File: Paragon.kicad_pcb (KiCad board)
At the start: 2 copper layers, 63 x 88 mm, 3 parts

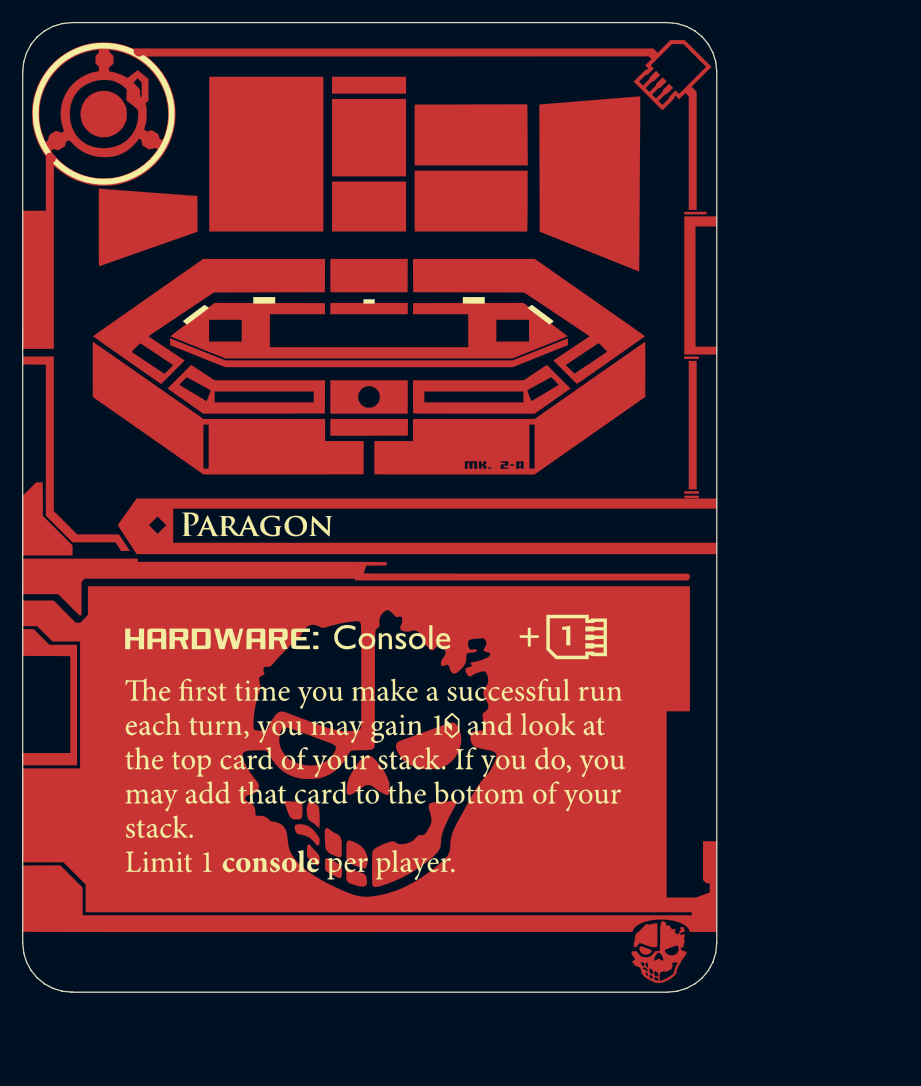
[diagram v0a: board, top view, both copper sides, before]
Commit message: Add files via upload
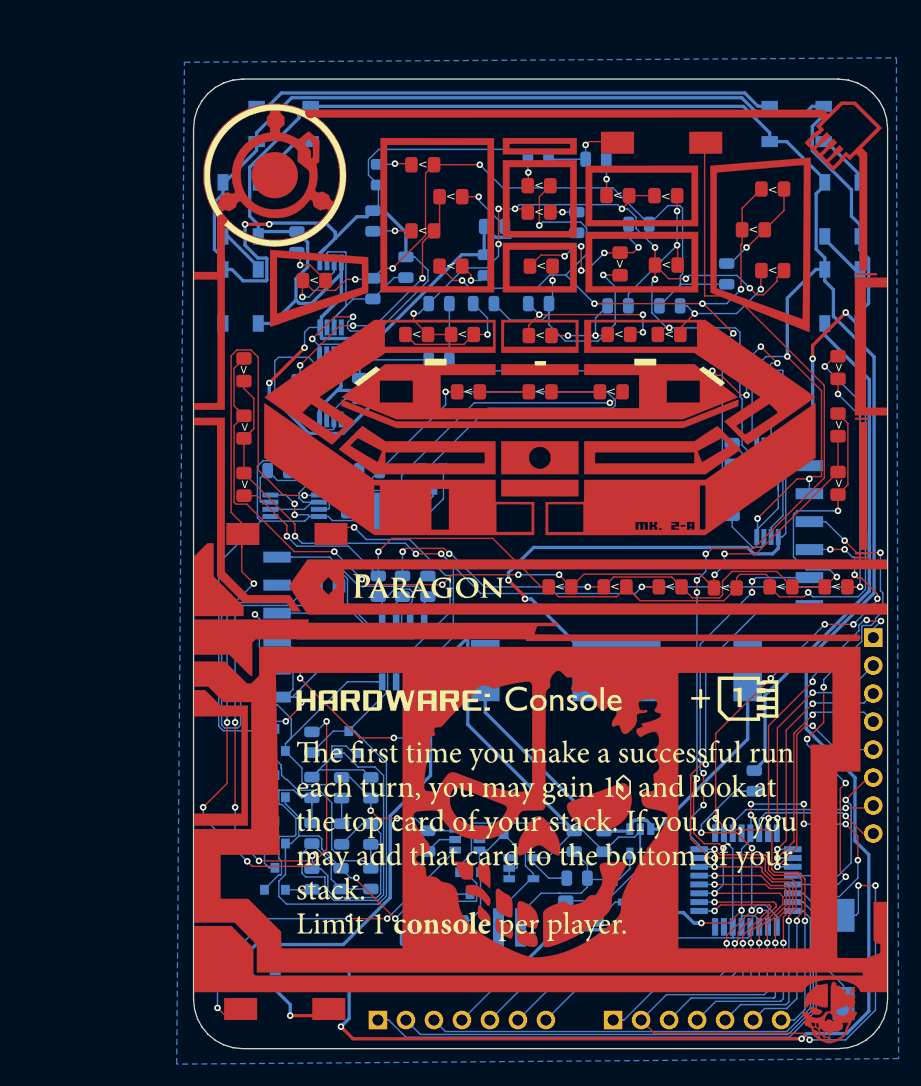
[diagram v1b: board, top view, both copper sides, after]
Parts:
- removed the G*** at (138.8, 93.2) (x2)
- removed the G*** at (138.8, 93.1)
- added 5551: NE555, Package_SO:TSSOP-8_4.4x3mm_P0.65mm, B.Cu at (135.3, 73.9)
- added 5552: NE555, Package_SO:TSSOP-8_4.4x3mm_P0.65mm, B.Cu at (135.2, 82.3)
- added 5553: NE555, Package_SO:TSSOP-8_4.4x3mm_P0.65mm, B.Cu at (174.9, 92.9)
- added 5554: NE555, Package_SO:TSSOP-8_4.4x3mm_P0.65mm, B.Cu at (174.9, 84.6)
- added AP2112: AP2112K-3.3, Package_TO_SOT_SMD:SOT-23-5, B.Cu at (163.0, 129.9)
- added ATA1: Conn_01x08_Male, KiCad Footprints:PinHeader_1x08_P2.54mm_Vertical, B.Cu at (184.5, 105.0)
- added ATD1: Conn_01x07_Male, KiCad Footprints:PinHeader_1x07_P2.54mm_Vertical, B.Cu at (139.6, 139.7)
- added ATD2: Conn_01x07_Male, KiCad Footprints:PinHeader_1x07_P2.54mm_Vertical, B.Cu at (160.9, 139.7)
- added ATM328: ATmega328P-AU, Package_QFP:TQFP-32_7x7mm_P0.8mm, B.Cu at (172.9, 127.0)
- added ATM328 SPI: Conn_01x06_Female, KiCad Footprints:ConnectorMicromatch-12, B.Cu at (178.7, 95.8)
- added ATT25: ATtiny25V-10SU, Package_SO:SOIC-8_3.9x4.9mm_P1.27mm, B.Cu at (141.8, 106.3)
- added ATTINY SPI: Conn_01x06_Female, KiCad Footprints:ConnectorMicromatch-12, B.Cu at (130.4, 104.0)
- added BT1: Battery 1.5 - 3V, Battery:BatteryHolder_MPD_BC2003_1x2032, B.Cu at (161.2, 108.0)
- added C1: CP1, Capacitor_SMD:C_0805_2012Metric, B.Cu at (138.9, 122.8)
- added C10: 10uf, Capacitor_SMD:C_0805_2012Metric, B.Cu at (145.1, 79.8)
- added C11: 10uf, Capacitor_SMD:C_0805_2012Metric, B.Cu at (142.1, 71.4)
- added C12: 10uf, Capacitor_SMD:C_0805_2012Metric, B.Cu at (137.9, 82.4)
- added C13: 10uf, Capacitor_SMD:C_0805_2012Metric, B.Cu at (171.7, 88.3)
- added C2: 470pF, Capacitor_SMD:C_0805_2012Metric, B.Cu at (138.8, 89.9)
- added C3: 1uf, Capacitor_SMD:C_0805_2012Metric, B.Cu at (156.6, 129.8)
- added C4: 1uf, Capacitor_SMD:C_0805_2012Metric, B.Cu at (159.4, 129.8)
- added C5: 10uf, Capacitor_SMD:C_0805_2012Metric, B.Cu at (157.4, 123.5)
- added C6: 68uf, Capacitor_SMD:C_0805_2012Metric, B.Cu at (147.1, 131.6)
- added C7: 33uf, Capacitor_SMD:C_0805_2012Metric, B.Cu at (160.1, 123.5)
- added C8: 33uf, Capacitor_SMD:C_0805_2012Metric, B.Cu at (157.6, 126.8)
- added D1: LED, KiCad Footprints:LED_0805_cardfront, B.Cu at (135.0, 100.3)
- added D10: LED, KiCad Footprints:LED_0805_cardfront, F.Cu at (154.2, 64.0)
- added D11: LED, KiCad Footprints:LED_0805_cardfront, F.Cu at (154.2, 66.4)
- added D12: LED, KiCad Footprints:LED_0805_cardfront, F.Cu at (161.3, 64.9)
- added D13: LED, KiCad Footprints:LED_0805_cardfront, F.Cu at (165.7, 64.9)
- added D14: LED, KiCad Footprints:LED_0805_cardfront, F.Cu at (165.7, 71.2)
- added D15: LED, KiCad Footprints:LED_0805_cardfront, F.Cu at (154.4, 71.3)
- added D16: LED, KiCad Footprints:LED_0805_cardfront, F.Cu at (161.5, 71.1)
- added D17: LED, KiCad Footprints:LED_0805_cardfront, F.Cu at (175.4, 64.3)
- added D18: LED, KiCad Footprints:LED_0805_cardfront, F.Cu at (173.6, 68.0)
- added D19: LED, KiCad Footprints:LED_0805_cardfront, F.Cu at (175.4, 71.7)
- added D2: LED, KiCad Footprints:LED_0805_cardfront, F.Cu at (160.7, 82.7)
- added D20: LED, KiCad Footprints:LED_0805_cardfront, F.Cu at (166.0, 77.5)
- added D21: LED, KiCad Footprints:LED_0805_cardfront, F.Cu at (154.3, 77.6)
- added D22: LED, KiCad Footprints:LED_0805_cardfront, F.Cu at (161.4, 77.5)
- added D23: LED, KiCad Footprints:LED_0805_cardfront, F.Cu at (143.1, 77.5)
- added D24: LED, KiCad Footprints:LED_0805_cardfront, F.Cu at (147.2, 77.5)
- added D25: LED, KiCad Footprints:LED_0805_cardfront, F.Cu at (181.1, 100.4)
- added D26: LED, KiCad Footprints:LED_0805_cardfront, F.Cu at (176.1, 100.4)
- added D27: LED, KiCad Footprints:LED_0805_cardfront, F.Cu at (171.1, 100.5)
- added D28: LED, KiCad Footprints:LED_0805_cardfront, F.Cu at (166.1, 100.4)
- added D29: LED, KiCad Footprints:LED_0805_cardfront, F.Cu at (161.1, 100.4)
- added D3: LED, KiCad Footprints:LED_0805_cardfront, F.Cu at (154.3, 82.7)
- added D30: LED, KiCad Footprints:LED_0805_cardfront, F.Cu at (156.1, 100.4)
- added D31: LED, KiCad Footprints:LED_0805_cardfront, F.Cu at (181.3, 91.0)
- added D32: LED, KiCad Footprints:LED_0805_cardfront, F.Cu at (181.3, 85.7)
- added D33: LED, KiCad Footprints:LED_0805_cardfront, F.Cu at (181.3, 80.5)
- added D34: LED, KiCad Footprints:LED_0805_cardfront, F.Cu at (127.4, 91.1)
- added D35: LED, KiCad Footprints:LED_0805_cardfront, F.Cu at (127.4, 85.9)
- added D36: LED, KiCad Footprints:LED_0805_cardfront, F.Cu at (127.4, 80.7)
- added D37: MBR0520LT, Diode_SMD:D_SOD-123, B.Cu at (152.6, 122.7)
- added D38: MBR0520LT, Diode_SMD:D_SOD-123, B.Cu at (162.5, 126.9)
- added D39: MBR0520LT, Diode_SMD:D_SOD-123, B.Cu at (135.3, 134.4)
- added D4: LED, KiCad Footprints:LED_0805_cardfront, F.Cu at (147.8, 82.7)
- added D40: WS2812B, LED_SMD:LED_WS2812B_PLCC4_5.0x5.0mm_P3.2mm, B.Cu at (181.7, 74.0)
- added D41: WS2812B, LED_SMD:LED_WS2812B_PLCC4_5.0x5.0mm_P3.2mm, B.Cu at (181.7, 66.2)
- added D42: WS2812B, LED_SMD:LED_WS2812B_PLCC4_5.0x5.0mm_P3.2mm, B.Cu at (177.6, 58.4)
- added D43: WS2812B, LED_SMD:LED_WS2812B_PLCC4_5.0x5.0mm_P3.2mm, B.Cu at (131.0, 58.4)
- added D44: WS2812B, LED_SMD:LED_WS2812B_PLCC4_5.0x5.0mm_P3.2mm, B.Cu at (127.1, 66.2)
- added D45: WS2812B, LED_SMD:LED_WS2812B_PLCC4_5.0x5.0mm_P3.2mm, B.Cu at (127.1, 74.0)
- added D5: LED, KiCad Footprints:LED_0805_cardfront, F.Cu at (133.8, 72.6)
- added D6: LED, KiCad Footprints:LED_0805_cardfront, F.Cu at (143.6, 62.1)
- added D7: LED, KiCad Footprints:LED_0805_cardfront, F.Cu at (146.2, 65.0)
- added D8: LED, KiCad Footprints:LED_0805_cardfront, F.Cu at (143.6, 68.1)
- added D9: LED, KiCad Footprints:LED_0805_cardfront, F.Cu at (146.2, 71.3)
- added G***: LOGO, KiCad Footprints:F_Cu, F.Cu at (154.3, 98.7)
- added G***: LOGO, KiCad Footprints:F_Mask, F.Cu at (154.3, 98.7)
- added G***: LOGO, KiCad Footprints:F_SilkS, F.Cu at (154.3, 98.7)
- added J1: Conn_01x02_Male, KiCad Footprints:Connector_2.54_2pin_SMD, B.Cu at (129.0, 134.4)
- added L1: L, KiCad Footprints:CD32_coil, B.Cu at (140.7, 93.6)
- added L2: 47uh, KiCad Footprints:CD32_coil, B.Cu at (151.5, 131.3)
- added LV555: ICM7555, Package_SO:VSSOP-8_3.0x3.0mm_P0.65mm, B.Cu at (132.0, 93.0)
- added MAX16054: MAX16054, Package_TO_SOT_SMD:SOT-23-6, B.Cu at (147.7, 123.3)
- added MAX40200: MAX40200, Package_TO_SOT_SMD:SOT-23-5, B.Cu at (163.4, 123.5)
- added NCP1402: NCP1402, Package_TO_SOT_SMD:SOT-23-5, B.Cu at (152.6, 125.9)
- added Q1: 2N3904, Package_TO_SOT_SMD:SOT-23, B.Cu at (130.2, 126.9)
- added Q2: 2N2222, Package_TO_SOT_SMD:SOT-23, B.Cu at (144.6, 90.6)
- added Q2A1: 2N3906, Package_TO_SOT_SMD:SOT-23, B.Cu at (130.2, 122.7)
- added Q2B1: 2N3906, Package_TO_SOT_SMD:SOT-23, B.Cu at (130.2, 118.5)
- added Q3: 2N3904, Package_TO_SOT_SMD:SOT-23, B.Cu at (130.2, 114.3)
- added Q4: 2N3904, Package_TO_SOT_SMD:SOT-23, B.Cu at (136.9, 114.5)
- added Q5: Si2301, Package_TO_SOT_SMD:SOT-23, B.Cu at (147.9, 127.3)
- added R1: 12, Resistor_SMD:R_0805_2012Metric, B.Cu at (133.6, 114.5)
- added R10: 1K, Resistor_SMD:R_0805_2012Metric, B.Cu at (136.9, 92.8)
- added R11: 1K, Resistor_SMD:R_0805_2012Metric, B.Cu at (130.5, 89.9)
- added R12: 10K, Resistor_SMD:R_0805_2012Metric, B.Cu at (134.7, 89.9)
- added R13: 75k, Resistor_SMD:R_0805_2012Metric, B.Cu at (139.1, 73.3)
- added R14: 68K, Resistor_SMD:R_0805_2012Metric, B.Cu at (132.4, 82.5)
- added R15: 62k, Resistor_SMD:R_0805_2012Metric, B.Cu at (171.7, 93.0)
- added R16: 56k, Resistor_SMD:R_0805_2012Metric, B.Cu at (145.1, 74.7)
- added R17: 200, Resistor_SMD:R_0805_2012Metric, B.Cu at (132.2, 69.1)
- added R18: 200, Resistor_SMD:R_0805_2012Metric, B.Cu at (139.6, 63.0)
- added R19: 200, Resistor_SMD:R_0805_2012Metric, B.Cu at (150.1, 67.7)
- added R2: 5.6K, Resistor_SMD:R_0805_2012Metric, B.Cu at (136.3, 122.8)
- added R20: 200, Resistor_SMD:R_0805_2012Metric, B.Cu at (139.1, 67.2)
- added R21: 200, Resistor_SMD:R_0805_2012Metric, B.Cu at (149.3, 71.2)
- added R22: 200, Resistor_SMD:R_0805_2012Metric, B.Cu at (154.1, 61.6)
- added R23: 200, Resistor_SMD:R_0805_2012Metric, B.Cu at (157.6, 67.3)
- added R24: 200, Resistor_SMD:R_0805_2012Metric, B.Cu at (159.3, 61.6)
- added R25: 200, Resistor_SMD:R_0805_2012Metric, B.Cu at (161.3, 74.9)
- added R26: 200, Resistor_SMD:R_0805_2012Metric, B.Cu at (163.2, 67.5)
- added R27: 200, Resistor_SMD:R_0805_2012Metric, B.Cu at (171.2, 72.0)
- added R28: 200, Resistor_SMD:R_0805_2012Metric, B.Cu at (166.0, 74.9)
- added R29: 200, Resistor_SMD:R_0805_2012Metric, B.Cu at (154.1, 74.7)
- added R3: 3.3k, Resistor_SMD:R_0805_2012Metric, B.Cu at (136.3, 118.6)
- added R30: 200, Resistor_SMD:R_0805_2012Metric, B.Cu at (149.1, 74.7)
- added R31: 100k, Resistor_SMD:R_0805_2012Metric, B.Cu at (143.0, 132.3)
- added R32: 33, Resistor_SMD:R_0805_2012Metric, B.Cu at (144.1, 100.3)
- added R33: 33, Resistor_SMD:R_0805_2012Metric, B.Cu at (142.6, 112.2)
- added R34: 33, Resistor_SMD:R_0805_2012Metric, B.Cu at (141.8, 100.3)
- added R35: 33, Resistor_SMD:R_0805_2012Metric, B.Cu at (139.6, 100.3)
- added R36: 100k, Resistor_SMD:R_0805_2012Metric, B.Cu at (144.1, 123.5)
- added R37: 220k, Resistor_SMD:R_0805_2012Metric, B.Cu at (173.7, 118.0)
- added R4: 410, Resistor_SMD:R_0805_2012Metric, B.Cu at (136.2, 126.9)
- added R5: 410, Resistor_SMD:R_0805_2012Metric, B.Cu at (138.9, 126.9)
- added R6: 22K, Resistor_SMD:R_0805_2012Metric, B.Cu at (133.6, 122.7)
- added R7: 10K, Resistor_SMD:R_0805_2012Metric, B.Cu at (133.6, 118.6)
- added R8: 22K, Resistor_SMD:R_0805_2012Metric, B.Cu at (138.9, 118.6)
- added R9: 100, Resistor_SMD:R_0805_2012Metric, B.Cu at (133.6, 126.9)
- added SW1: SW_Push, KiCad Footprints:SMD_button, F.Cu at (131.1, 138.7)
- added SW2: SW_Push, KiCad Footprints:SMD_button, F.Cu at (131.3, 95.6)
- added SW3: SW_Push, KiCad Footprints:SMD_button, B.Cu at (181.8, 134.2)
- added SW4: SW_Push, KiCad Footprints:SMD_button, F.Cu at (165.3, 60.1)
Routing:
- net Earth: track 0.00 -> 462.5 mm, vias 0 -> 18
- net Net-(AP2112-Pad1): track 0.00 -> 412.5 mm, vias 0 -> 7
- net Net-(ATT25-Pad8): track 0.00 -> 161.6 mm, vias 0 -> 7
- net Net-(ATT25-Pad4): track 0.00 -> 160.4 mm, vias 0 -> 5
- net Net-(ATD2-Pad1): track 0.00 -> 115.4 mm, vias 0 -> 7
- net Net-(D25-Pad2): track 0.00 -> 111.1 mm, vias 0 -> 6
- net Net-(D26-Pad1): track 0.00 -> 94.1 mm, vias 0 -> 4
- net Net-(D10-Pad2): track 0.00 -> 90.1 mm, vias 0 -> 8
- net Net-(D11-Pad1): track 0.00 -> 84.9 mm, vias 0 -> 10
- net Net-(D27-Pad1): track 0.00 -> 84.6 mm, vias 0 -> 7
- net Net-(ATD2-Pad2): track 0.00 -> 70.5 mm, vias 0 -> 5
- net Net-(D25-Pad1): track 0.00 -> 69.5 mm, vias 0 -> 5
- net Net-(D5-Pad1): track 0.00 -> 66.0 mm, vias 0 -> 4
- net Net-(ATD2-Pad7): track 0.00 -> 65.1 mm, vias 0 -> 9
- net Net-(ATD2-Pad6): track 0.00 -> 59.3 mm, vias 0 -> 6
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- added copper zone on B.Cu, net Earth
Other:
- net class Default: clearance 0.2 -> 0.13; trace_width 0.25 -> 0.13; via_dia 0.8 -> 0.6; via_drill 0.4 -> 0.3
- net class RGB Power added: clearance 0.13, trace_width 0.3, via_dia 0.6, via_drill 0.3
- rule pad_to_mask_clearance: 0.2 -> 0
- rule trace_clearance: 0.2 -> 0.13
- rule trace_min: 0.2 -> 0.13
- rule via_min_size: 0.4 -> 0.6
- board text added: "0"
- board text added: "1"
- board text added: "10"
- board text added: "11"
- board text added: "12"
- board text added: "13"
- board text added: "2"
- board text added: "3"
- board text added: "4"
- board text added: "5"
- board text added: "6"
- board text added: "7"
- board text added: "8"
- board text added: "9"
- board text added: "A0"
- board text added: "A1"
- board text added: "A2"
- board text added: "A3"
- board text added: "A4"
- board text added: "A5"
- board text added: "A6"
- board text added: "A7"
- board text added: "GND"
- board text added: "MISO"
- board text added: "MOSI"
- board text added: "RESET"
- board text added: "SCK"
- board text added: "VCC"
- board text added: "github.com/timbalicious"
